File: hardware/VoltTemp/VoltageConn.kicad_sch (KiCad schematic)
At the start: 26 parts, among them J1 Conn_01x11, J7 Conn_01x04

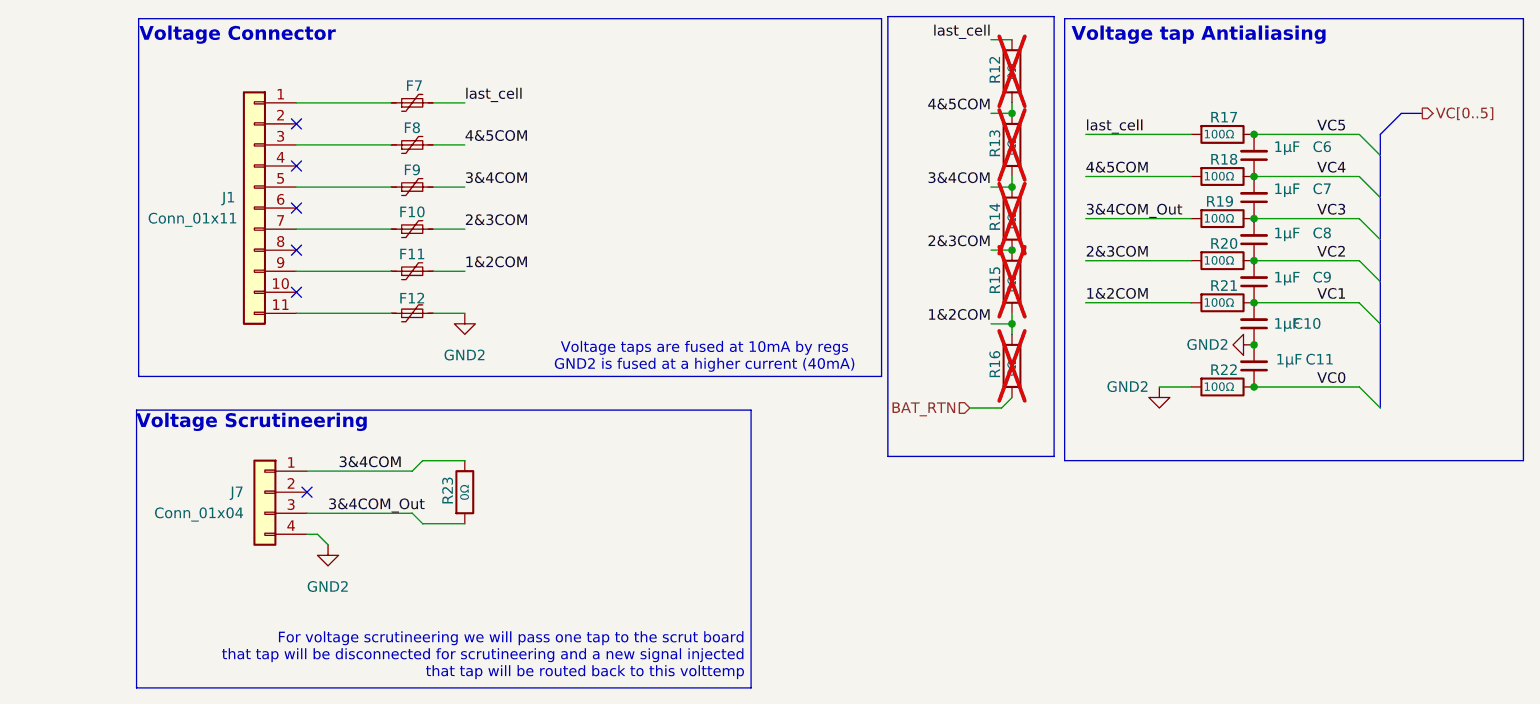
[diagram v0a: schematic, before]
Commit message: schematic mostly done
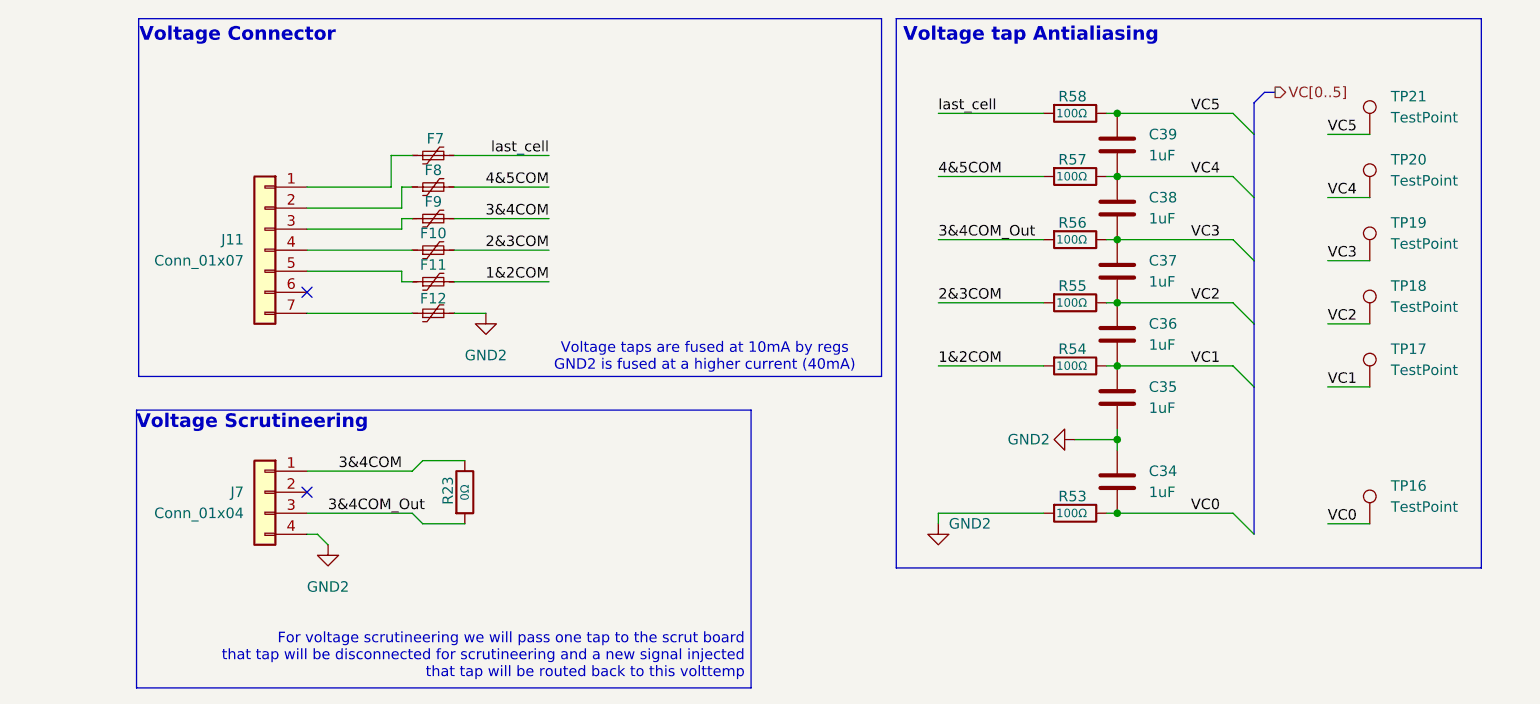
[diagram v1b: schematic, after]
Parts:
- removed C10, C11, C6, C7, C8, C9: 1μF, Capacitor_SMD:C_0805_2012Metric, symbol Device:C_Small
- removed J1: Conn_01x11, symbol Connector_Generic:Conn_01x11
- removed R12, R13, R14, R15, R16: 0Ω, Resistor_SMD:R_0805_2012Metric, symbol Device:R
- removed R17, R18, R19, R20, R21, R22: 100Ω, Resistor_SMD:R_0805_2012Metric, symbol Device:R
- added C34, C35, C36, C37, C38, C39: 1uF, Capacitor_SMD:C_0603_1608Metric_Pad1.08x0.95mm_HandSolder, symbol Device:C
- added J11: Conn_01x07, VoltTemp:1053131107, symbol Connector_Generic:Conn_01x07
- added R53, R54, R55, R56, R57, R58: 100Ω, Resistor_SMD:R_0603_1608Metric_Pad0.98x0.95mm_HandSolder, symbol Device:R
- added TP16, TP17, TP18, TP19, TP20, TP21: TestPoint, TestPoint:TestPoint_Pad_1.5x1.5mm, symbol Connector:TestPoint
- F10, F11, F12, F7, F8, F9: footprint UTSVT_Special:ptc_fuse_FUSC1607X75N -> VoltTemp:ptc_fuse_FUSC1607X75N
- J7: footprint (none) -> VoltTemp:1053132104; P/N (none) -> 1053132104
- R23: footprint Resistor_SMD:R_0805_2012Metric -> Resistor_SMD:R_0603_1608Metric_Pad0.98x0.95mm_HandSolder; P/N SMD_0805 -> (none)
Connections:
- net 1&2COM: now also R54.2
- net 2&3COM: now also R55.2
- net 3&4COM_Out: now also R56.2
- net 4&5COM: now also R57.2
- net GND2: now also C34.1, C35.2, R53.2
- net VC0: now also C34.2, R53.1, TP16.1
- net VC1: now also C35.1, C36.2, R54.1, TP17.1
- net VC2: now also C36.1, C37.2, R55.1, TP18.1
- net VC3: now also C37.1, C38.2, R56.1, TP19.1
- net VC4: now also C38.1, C39.2, R57.1, TP20.1
- net VC5: now also C39.1, R58.1, TP21.1
- net last_cell: now also R58.2
- net at F8.1: now also J11.2 (Pin_2)
- net at F11.1: now also J11.5 (Pin_5)
- net at F10.1: now also J11.4 (Pin_4)
- net at F7.1: now also J11.1 (Pin_1)
- net at F12.1: now also J11.7 (Pin_7)
- net at F9.1: now also J11.3 (Pin_3)
- no-connect marks 6 -> 2
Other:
- moved on the sheet: F10, F11, F12, F7, F8, F9
